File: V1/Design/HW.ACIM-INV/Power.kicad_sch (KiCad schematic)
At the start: 91 parts, among them J1 AC POWER INPUT, M4 470V/1.2kA, M5 470V/1.2kA, M6 470V/1.2kA, M7 470V/1.2kA, Q10 20V/1A, Q11 20V/1A, U10 SMPS 5V±2%/1.5A, U13 LDO 3.3V±0.5%/1A, U14 SMPS 24V±2%/1A, U17 LDO 5V±0.4%/250mA

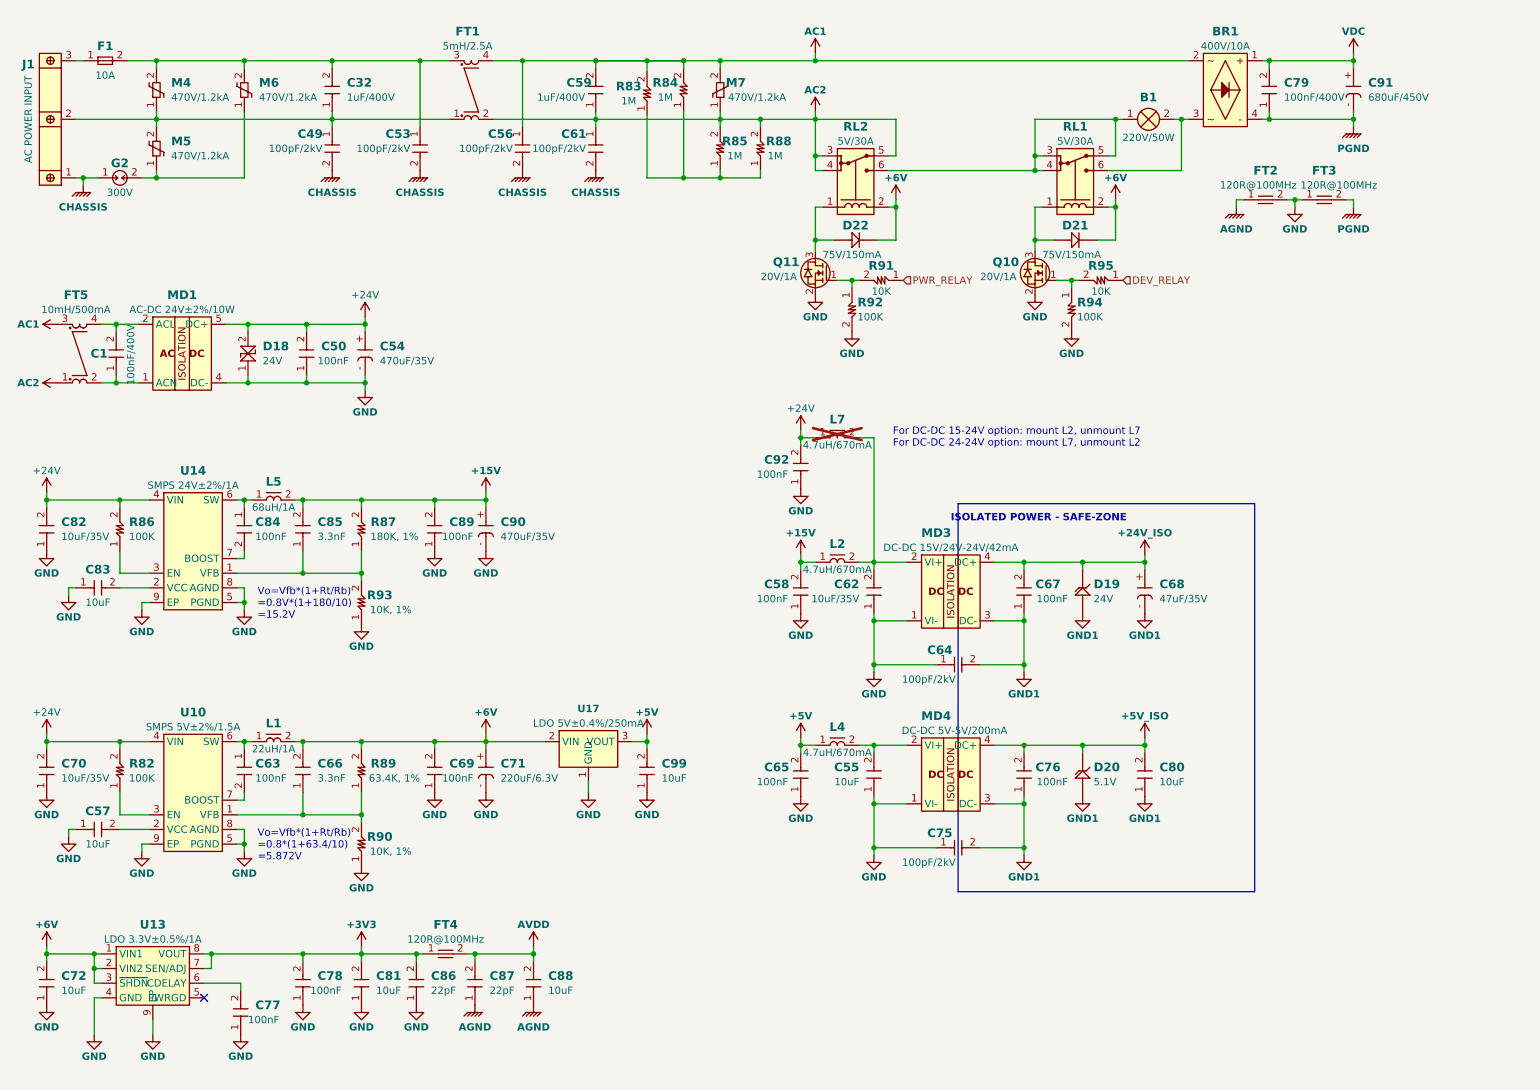
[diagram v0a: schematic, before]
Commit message: V1 schematic update 7
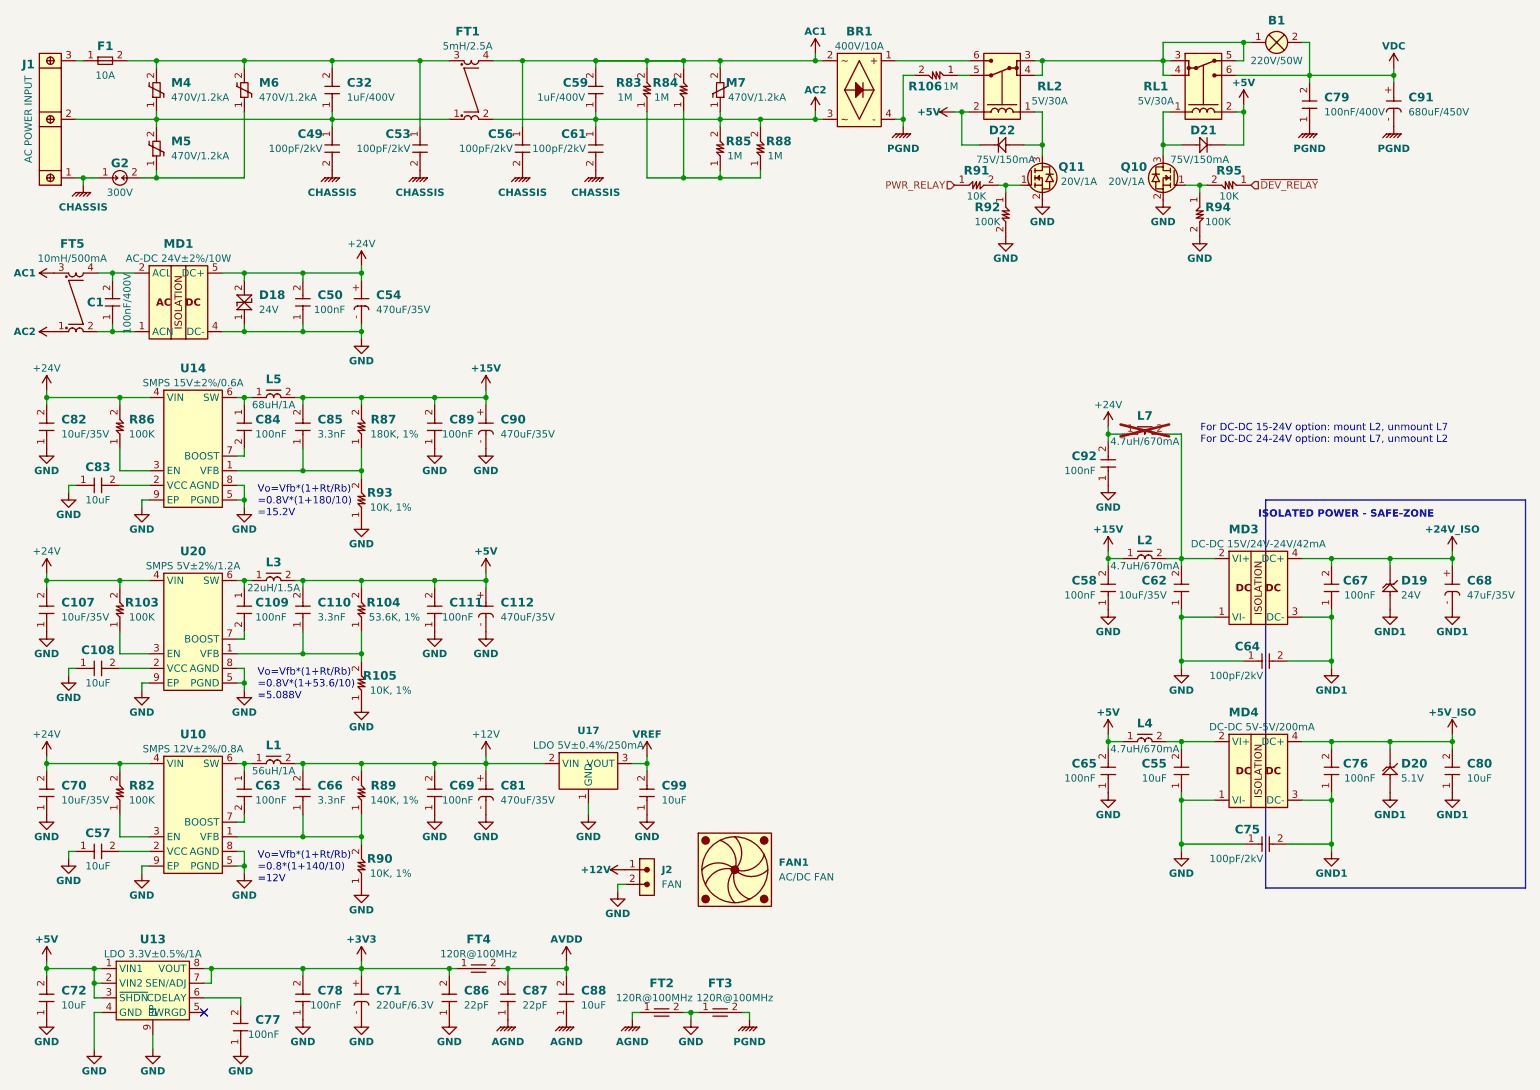
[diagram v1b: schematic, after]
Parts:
- removed C81: 10uF, SAMPI:CAP0603, symbol SAMPI:CERCAP
- added C107: 10uF/35V, SAMPI:CAP0603, symbol SAMPI:CERCAP
- added C108: 10uF, SAMPI:CAP0603, symbol SAMPI:CERCAP
- added C109, C111: 100nF, SAMPI:CAP0603, symbol SAMPI:CERCAP
- added C110: 3.3nF, SAMPI:CAP0603, symbol SAMPI:CERCAP
- added C112, C81: 470uF/35V, SAMPI:CAP_ELEC-10.3x10.3-DIA10, symbol SAMPI:ELECCAP
- added FAN1: AC/DC FAN, symbol SAMPI:FAN
- added J2: FAN, SAMPI:HDM-2x2.54-TH, symbol SAMPI:SIL02-2
- added L3: 22uH/1.5A, SAMPI:IND-8D43-8045, symbol SAMPI:IND
- added R103: 100K, SAMPI:RES0603, symbol SAMPI:RES
- added R104: 53.6K, 1%, SAMPI:RES0603, symbol SAMPI:RES
- added R105: 10K, 1%, SAMPI:RES0603, symbol SAMPI:RES
- added R106: 1M, SAMPI:RES1206, symbol SAMPI:RES
- added U20: SMPS 5V±2%/1.2A, SAMPI:TDFN8_2x3_MCHP, symbol SAMPI:MCP16311-TDFN
- D18: footprint SAMPI:DO-214AA -> SAMPI:DO-214AA-12
- FT1: footprint SAMPI:ToroidCoil-3119-13-D1 -> SAMPI:IND-SQ1010; MFT DIY -> OEM; MNP CUSTOM 1 -> SQ1010-5MH
- L1: value 22uH/1A -> 56uH/1A
- R89: value 63.4K, 1% -> 140K, 1%
- U10: value SMPS 5V±2%/1.5A -> SMPS 12V±2%/0.8A
- U14: value SMPS 24V±2%/1A -> SMPS 15V±2%/0.6A
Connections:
- net +24V: now also C107.2, R103.2, U20.4 (VIN)
- net +3V3: now also C71.+
- net +5V: now also C72.2, D21.K, D22.K, RL1.2 (COIL2), RL2.2 (COIL2), U13.1 (VIN1), U13.2 (VIN2), U13.3 (~{SHDN}), C110.2, C111.2, C112.+, L3.2, R104.2; no longer C99.2, U17.3 (VOUT)
- net AC2: now also BR1.3 (AC2); no longer RL2.3 (COM), RL2.4 (COM), RL2.5 (NC)
- net GND: now also C107.1, C108.1, C111.1, C112.-, C81.-, J2.2, R105.1, U20.5 (PGND), U20.8 (AGND), U20.9 (EP)
- net PGND: now also R106.2
- net VDC: now also B1.2, RL1.6 (NO); no longer BR1.1 (DC+)
- net at B1.1, RL1.3 (COM), RL1.4 (COM)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: now also RL2.3 (COM), RL2.4 (COM); no longer RL2.6 (NO)
- removed net +6V: C66.2, C69.2, C71.+, C72.2, D21.K, D22.K, L1.2, R89.2, RL1.2 (COIL2), RL2.2 (COIL2), U13.1 (VIN1), U13.2 (VIN2), U13.3 (~{SHDN}), U17.2 (VIN)
- net DEV_RELAY renamed ~{DEV_RELAY}
- new net: C110.1, R104.1, R105.2, U20.1 (VFB)
- new net: C108.2, U20.2 (VCC)
- new net: R106.1, RL2.5 (NC)
- new net: BR1.1 (DC+), RL2.6 (NO)
- new net: R103.1, U20.3 (EN)
- new net: C109.1, L3.1, U20.6 (SW)
- new net: C109.2, U20.7 (BOOST)
- new net +12V: C66.2, C69.2, C81.+, J2.1, L1.2, R89.2, U17.2 (VIN)
- new net VREF: C99.2, U17.3 (VOUT)
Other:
- moved on the sheet: B1, BR1, C1, C50, C54, C55, C57, C58, C62, C63, C64, C65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
